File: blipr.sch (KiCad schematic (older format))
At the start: 2 parts

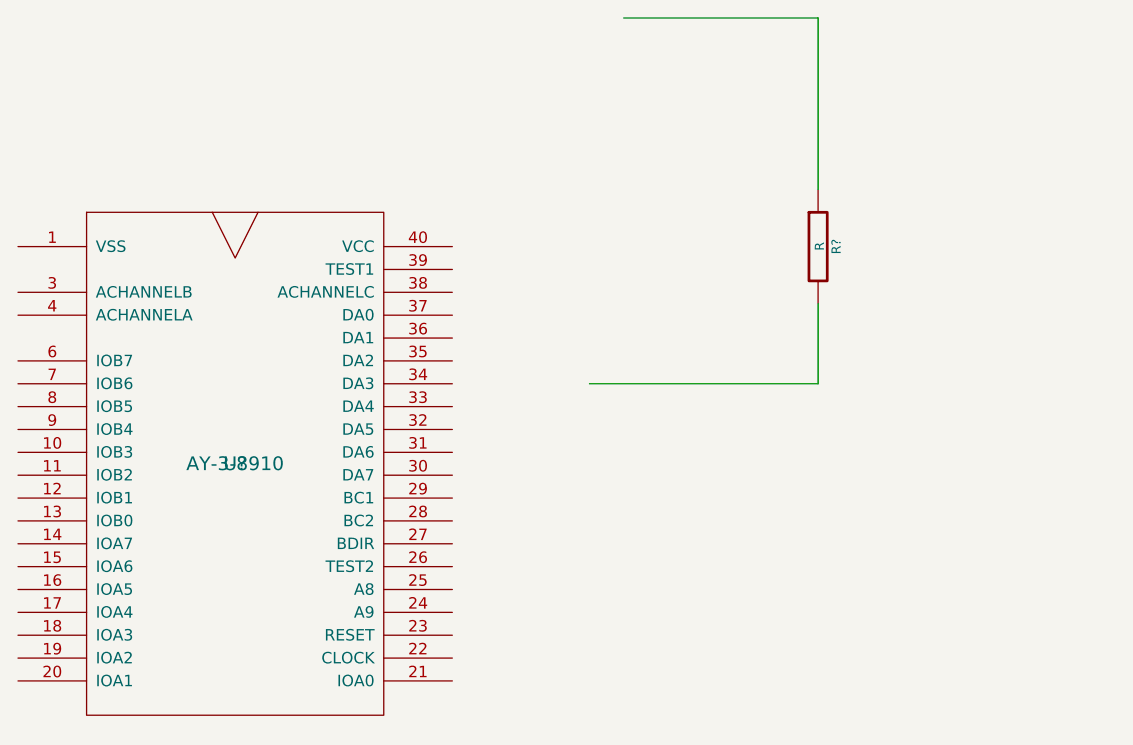
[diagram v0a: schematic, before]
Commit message: Hej
hej
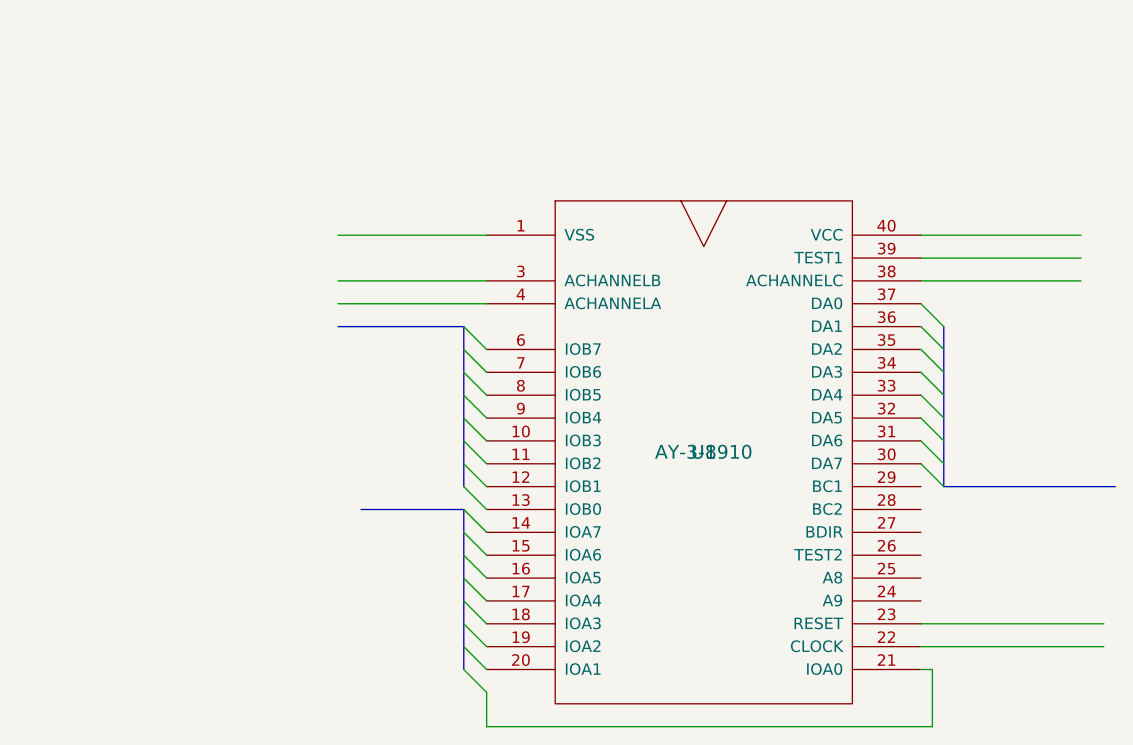
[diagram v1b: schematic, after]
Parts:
- removed R?: R, ~, symbol R
- gave numbers to parts that had none: 1
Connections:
- wire segments 4 -> 12
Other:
- moved on the sheet: U1
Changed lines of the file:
@@
-EESchema Schematic File Version 2  date 02/03/2014 18:52:32
+EESchema Schematic File Version 2  date 02/03/2014 19:15:03
 LIBS:power
 LIBS:device
@@
 $EndDescr
 $Comp
-L R R?
-U 1 1 53136D33
-P 7000 2950
-F 0 "R?" V 7080 2950 40  0000 C CNN
-F 1 "R" V 7007 2951 40  0000 C CNN
-F 2 "~" V 6930 2950 30  0000 C CNN
-F 3 "~" H 7000 2950 30  0000 C CNN
-	1    7000 2950
+L AY-3-8910 U1
+U 1 1 53136FF6
+P 6500 3850
+F 0 "U1" H 6500 3850 60  0000 C CNN
+F 1 "AY-3-8910" H 6500 3850 60  0000 C CNN
+F 2 "~" H 6500 3850 60  0000 C CNN
+F 3 "~" H 6500 3850 60  0000 C CNN
+	1    6500 3850
 	1    0    0    -1
 $EndComp
 Wire Wire Line
-	7000 2700 7000 1950
+	5550 2900 4900 2900
 Wire Wire Line
-	7000 1950 6150 1950
+	7450 2900 8150 2900
+Entry Wire Line
+	7450 3500 7550 3600
+Wire Bus Line
+	7550 4000 8300 4000
+Entry Wire Line
+	7450 3400 7550 3500
+Entry Wire Line
+	7450 3300 7550 3400
+Entry Wire Line
+	7450 3200 7550 3300
+Entry Wire Line
+	7450 3600 7550 3700
+Entry Wire Line
+	7450 3700 7550 3800
+Entry Wire Line
+	7450 3800 7550 3900
+Entry Wire Line
+	7450 3900 7550 4000
+Wire Bus Line
+	7550 4000 7550 3300
+Entry Wire Line
+	5450 3400 5550 3500
+Entry Wire Line
+	5450 3800 5550 3900
+Entry Wire Line
+	5450 3900 5550 4000
+Entry Wire Line
+	5450 4000 5550 4100
+Entry Wire Line
+	5450 4200 5550 4300
+Entry Wire Line
+	5450 4300 5550 4400
+Entry Wire Line
+	5450 4500 5550 4600
+Entry Wire Line
+	5450 4600 5550 4700
+Entry Wire Line
+	5450 4700 5550 4800
+Wire Bus Line
+	5450 4100 5450 4800
+Wire Bus Line
+	5450 4100 5000 4100
+Wire Bus Line
+	5450 4000 5450 3300
+Wire Bus Line
+	5450 3300 4900 3300
+Entry Wire Line
+	5450 3300 5550 3400
+Entry Wire Line
+	5450 3500 5550 3600
+Entry Wire Line
+	5450 3600 5550 3700
+Entry Wire Line
+	5450 3700 5550 3800
+Entry Wire Line
+	5450 4100 5550 4200
+Entry Wire Line
+	5450 4400 5550 4500
 Wire Wire Line
-	7000 3200 7000 3550
+	7450 4600 8250 4600
 Wire Wire Line
-	7000 3550 6000 3550
-$Comp
-L AY-3-8910 U?
-U 1 1 53136FF6
-P 4450 3900
-F 0 "U?" H 4450 3900 60  0000 C CNN
-F 1 "AY-3-8910" H 4450 3900 60  0000 C CNN
-F 2 "~" H 4450 3900 60  0000 C CNN
-F 3 "~" H 4450 3900 60  0000 C CNN
-	1    4450 3900
-	1    0    0    -1
-$EndComp
+	7450 4700 8250 4700
+Wire Wire Line
+	7450 4800 7500 4800
+Wire Wire Line
+	7500 4800 7500 5050
+Wire Wire Line
+	7500 5050 5550 5050
+Wire Wire Line
+	5550 5050 5550 4900
+Entry Wire Line
+	5450 4800 5550 4900
+Wire Wire Line
+	5550 3100 4900 3100
+Wire Wire Line
+	5550 3200 4900 3200
+Wire Wire Line
+	7450 3000 8150 3000
+Wire Wire Line
+	7450 3100 8150 3100
 $EndSCHEMATC
